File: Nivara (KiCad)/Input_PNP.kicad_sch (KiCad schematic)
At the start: 8 parts

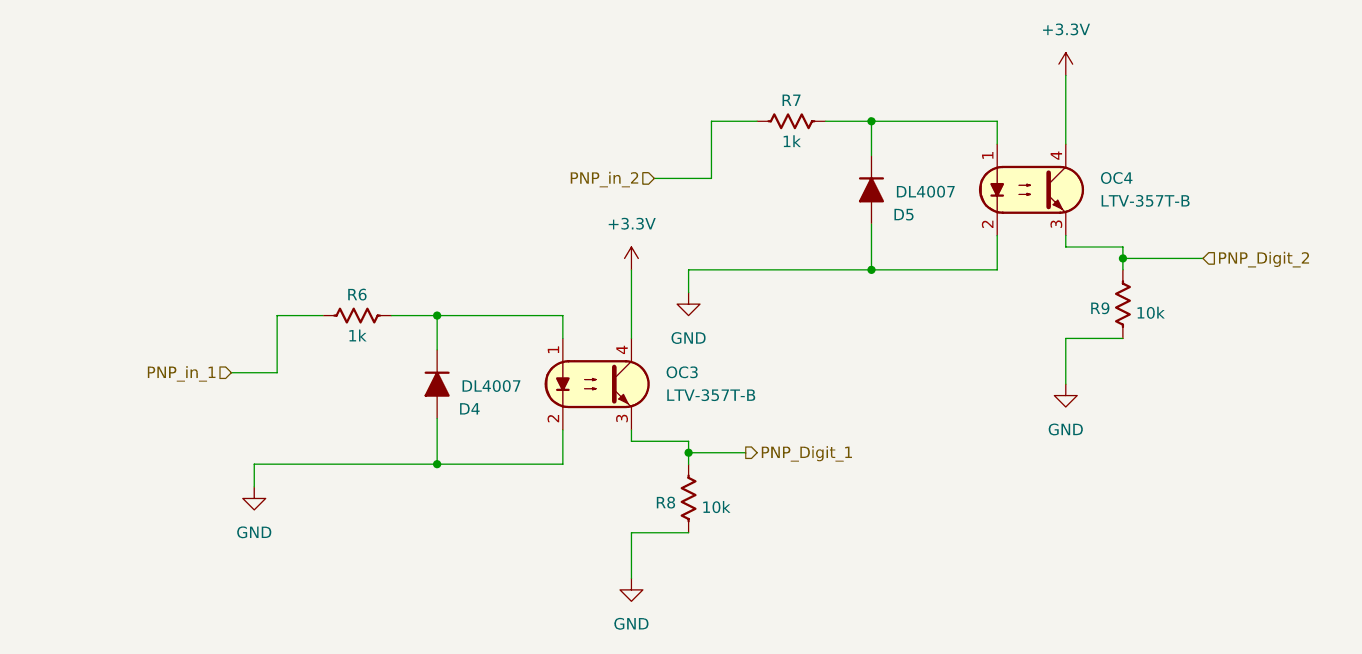
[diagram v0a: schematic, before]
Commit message: Add files via upload
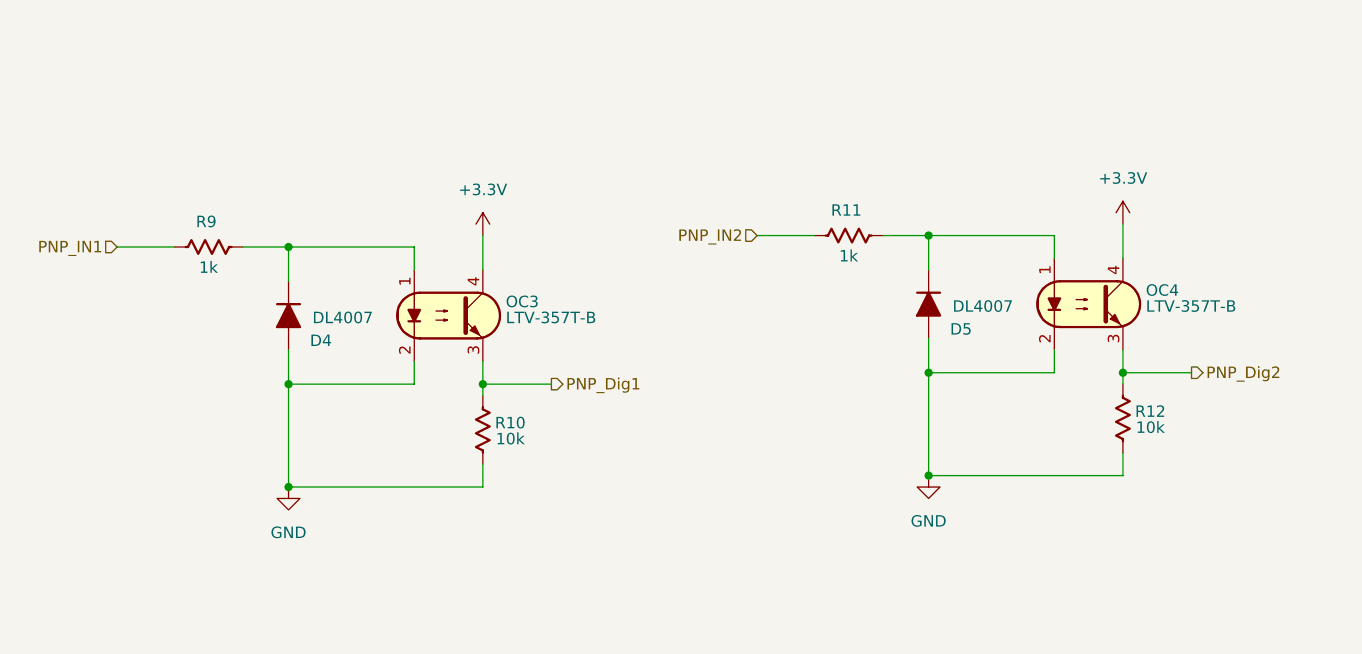
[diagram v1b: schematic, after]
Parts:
- removed R6, R7, R8: R_0603, PCM_Resistor_SMD_AKL:R_0603_1608Metric, symbol PCM_Resistor_US_AKL:R_0603
- added R10, R11, R12: R_0603, Resistor_SMD:R_0603_1608Metric, symbol PCM_Resistor_US_AKL:R_0603
- OC3, OC4: footprint PCM_Package_SO_AKL:SO-4_4.4x3.9mm_P2.54mm -> Package_SO:SO-4_4.4x2.3mm_P1.27mm
- R9: footprint PCM_Resistor_SMD_AKL:R_0603_1608Metric -> Resistor_SMD:R_0603_1608Metric; Capacidad 10k -> 1k
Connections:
- net GND: now also R10.2, R12.2; no longer R9.2
- net at D4.1 (K), OC3.1: now also R9.2
- net at D5.1 (K), OC4.1: now also R11.2
- net PNP_Digit_1 renamed PNP_Dig1
- net PNP_Dig1: now also R10.1
- net PNP_Digit_2 renamed PNP_Dig2
- net PNP_Dig2: now also R12.1; no longer R9.1
- new net PNP_IN1: R9.1
- new net PNP_IN2: R11.1
